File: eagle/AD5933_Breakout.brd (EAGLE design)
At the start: 22.9 x 20.3 mm, 5 parts, among them U1 AD5933

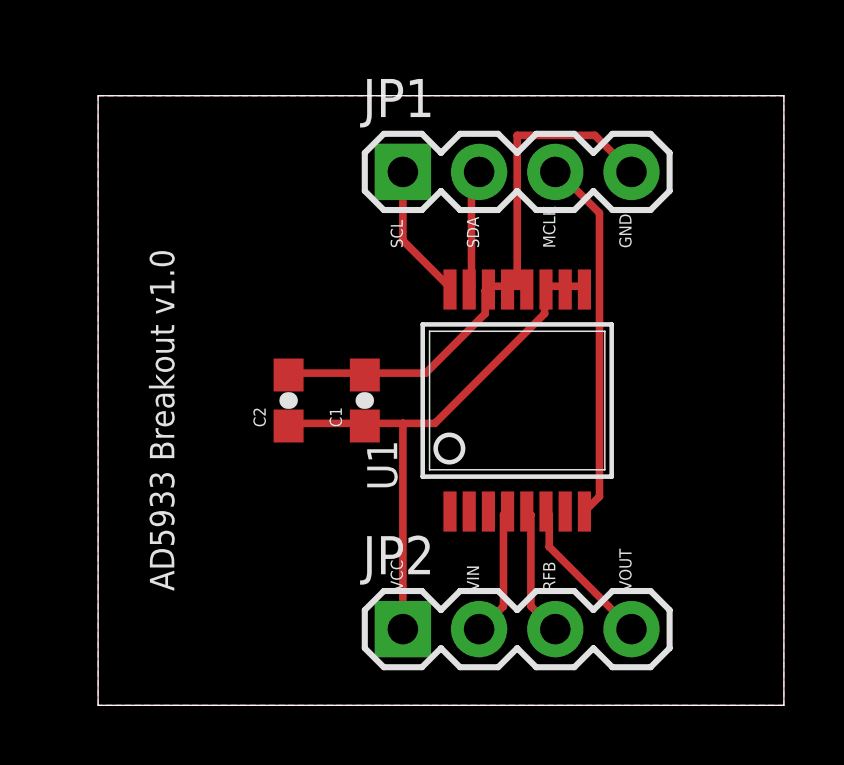
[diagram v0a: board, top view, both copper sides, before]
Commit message: created new gerber files
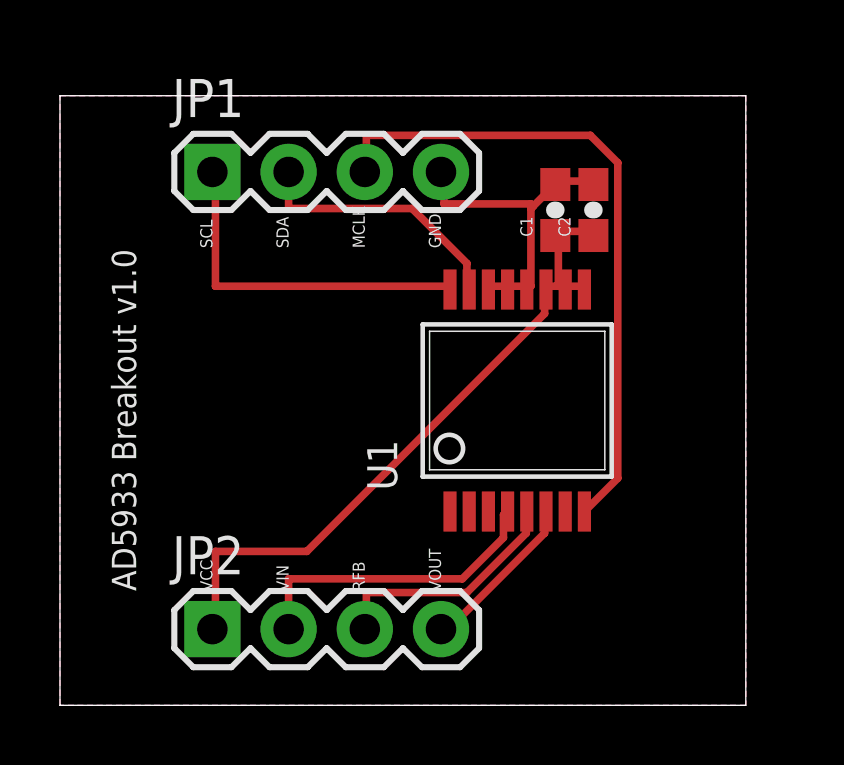
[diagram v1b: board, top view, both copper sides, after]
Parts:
- moved C2 12.0 mm to (21.6, 17.8)
- moved C1 8.98 mm to (20.3, 17.8)
- moved JP1 6.35 mm to (8.89, 19.1)
- moved JP2 6.35 mm to (8.89, 3.81)
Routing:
- net MCLK: track 12.2 -> 22.1 mm
- net GND: track 19.3 -> 11.0 mm
- net SCL: track 4.56 -> 11.8 mm
- net RFB: track 4.35 -> 10.3 mm
- net SDA: track 4.11 -> 8.82 mm
- net VIN: track 4.35 -> 8.15 mm
- net VCC: track 19.4 -> 22.5 mm
